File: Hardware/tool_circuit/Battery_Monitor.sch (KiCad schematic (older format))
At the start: 1 part

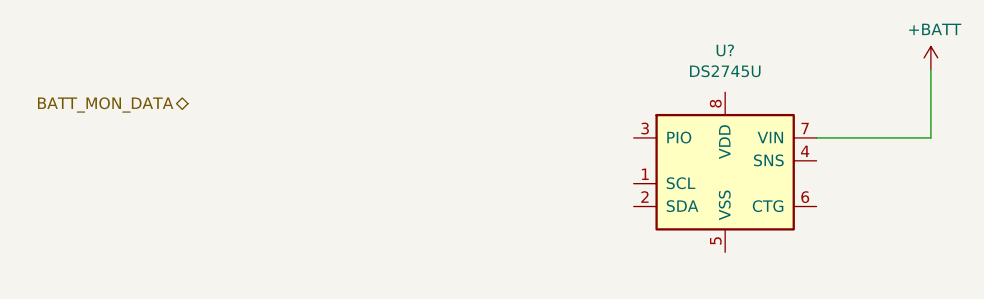
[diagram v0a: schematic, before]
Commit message: regulator/other changes
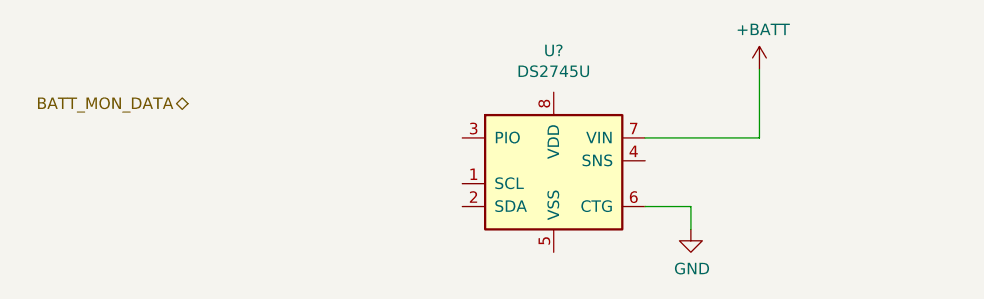
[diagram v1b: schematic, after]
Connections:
- net GND: now reaches U?.6 (CTG)
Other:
- moved on the sheet: U?
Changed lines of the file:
@@
 $Descr A4 11693 8268
 encoding utf-8
-Sheet 3 6
+Sheet 3 7
 Title ""
 Date ""
@@
 L Battery_Management:DS2745U U?
 U 1 1 611EC761
-P 7400 3450
+P 6650 3450
 AR Path="/611EC761" Ref="U?"  Part="1"
 AR Path="/611DF2F9/611EC761" Ref="U?"  Part="1"
-F 0 "U?" H 7400 3931 50  0000 C CNN
-F 1 "DS2745U" H 7400 3840 50  0000 C CNN
-F 2 "Package_SO:TSSOP-8_3x3mm_P0.65mm" H 7400 2950 50  0001 C CNN
-F 3 "https://datasheets.maximintegrated.com/en/ds/DS2745.pdf" H 7500 3050 50  0001 C CNN
-	1    7400 3450
+F 0 "U?" H 6650 3931 50  0000 C CNN
+F 1 "DS2745U" H 6650 3840 50  0000 C CNN
+F 2 "Package_SO:TSSOP-8_3x3mm_P0.65mm" H 6650 2950 50  0001 C CNN
+F 3 "https://datasheets.maximintegrated.com/en/ds/DS2745.pdf" H 6750 3050 50  0001 C CNN
+	1    6650 3450
 	1    0    0    -1
 $EndComp
@@
 L power:+BATT #PWR?
 U 1 1 611ED520
-P 8300 3050
-F 0 "#PWR?" H 8300 2900 50  0001 C CNN
-F 1 "+BATT" H 8315 3223 50  0000 C CNN
-F 2 "" H 8300 3050 50  0001 C CNN
-F 3 "" H 8300 3050 50  0001 C CNN
-	1    8300 3050
+P 7550 3050
+F 0 "#PWR?" H 7550 2900 50  0001 C CNN
+F 1 "+BATT" H 7565 3223 50  0000 C CNN
+F 2 "" H 7550 3050 50  0001 C CNN
+F 3 "" H 7550 3050 50  0001 C CNN
+	1    7550 3050
 	1    0    0    -1
 $EndComp
 Wire Wire Line
-	8300 3050 8300 3350
+	7550 3050 7550 3350
 Wire Wire Line
-	8300 3350 7800 3350
+	7550 3350 7050 3350
+$Comp
+L power:GND #PWR?
+U 1 1 612D54EC
+P 7250 3750
+F 0 "#PWR?" H 7250 3500 50  0001 C CNN
+F 1 "GND" H 7255 3577 50  0000 C CNN
+F 2 "" H 7250 3750 50  0001 C CNN
+F 3 "" H 7250 3750 50  0001 C CNN
+	1    7250 3750
+	1    0    0    -1
+$EndComp
+Wire Wire Line
+	7050 3650 7250 3650
+Wire Wire Line
+	7250 3650 7250 3750
 $EndSCHEMATC
